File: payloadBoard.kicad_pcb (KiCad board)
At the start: 4 copper layers, 20 x 45 mm, 49 parts, among them J1 USB_C_Receptacle_USB2.0_16P, J2 SERVO, J3 2S Battery, J4 Conn_01x04, U1 nRF52833_QDxx, U2 AT25SF041-SSHB-X, U3 LSM6DSO32, U4 AP63205WU, U5 AP63203WU, Y2 Crystal_GND24

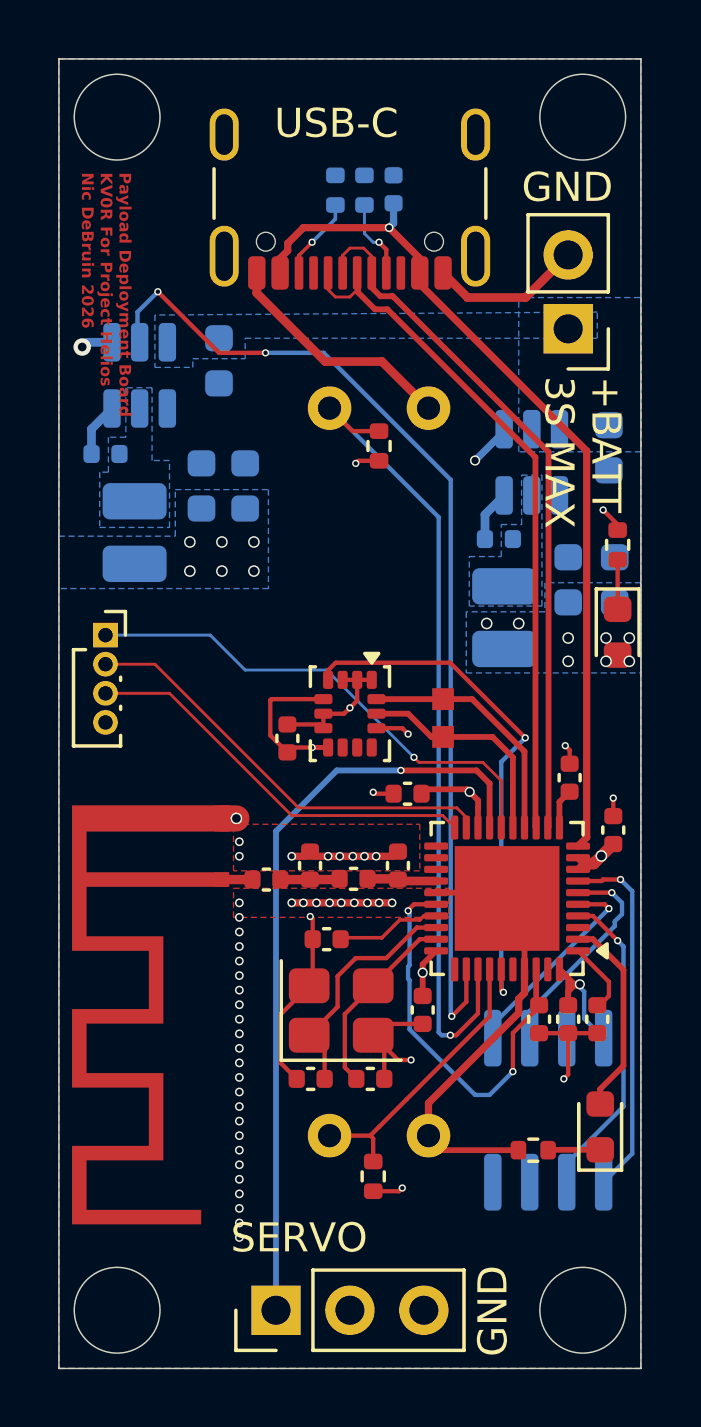
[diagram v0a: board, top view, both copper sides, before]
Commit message: board done, plenty small
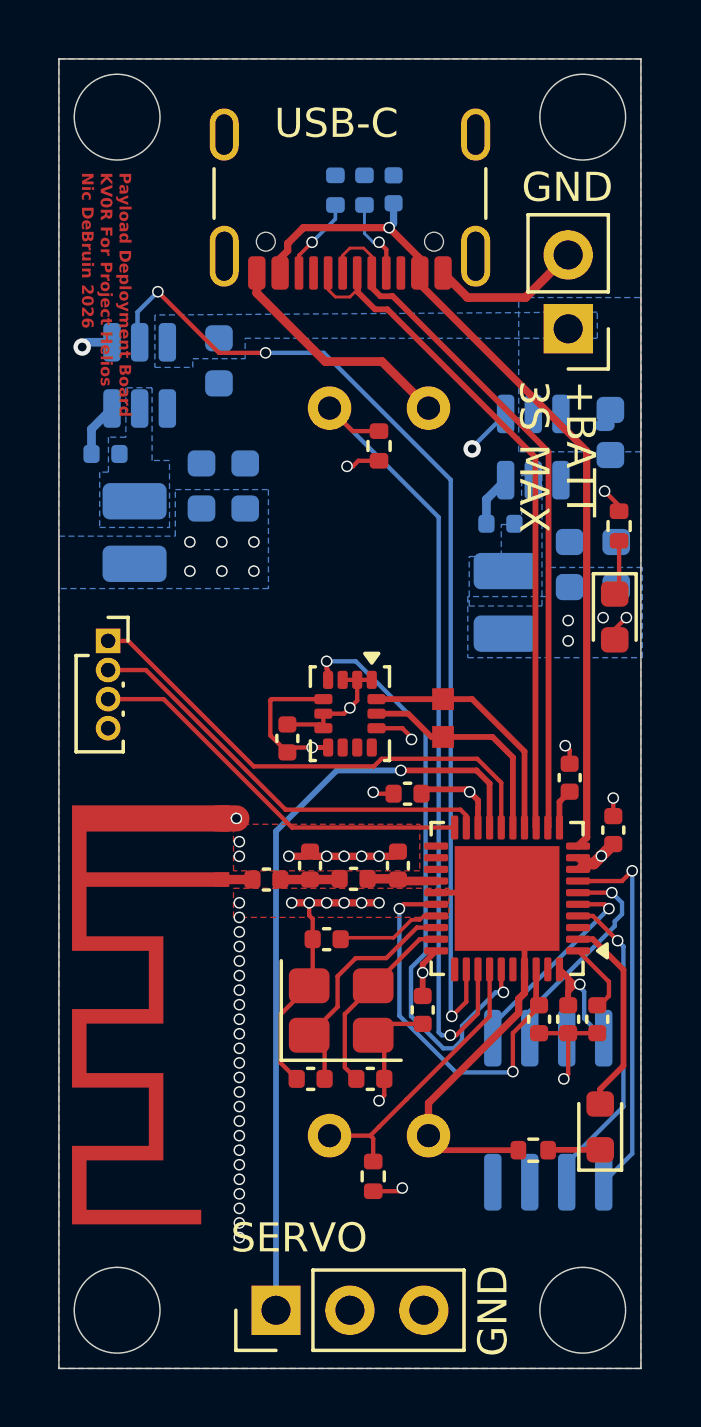
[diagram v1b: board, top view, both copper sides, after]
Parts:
- moved R7 0.65 mm to (164.2, 81.1)
- moved D1 0.53 mm to (164.1, 84.2)
- moved C20 0.53 mm to (164.2, 82.4)
- moved C21 0.53 mm to (162.6, 82.4)
- moved C19 0.53 mm to (160.2, 81.0)
- moved L4 0.53 mm to (160.3, 83.7)
- moved U5 0.53 mm to (161.3, 78.3)
- moved C18 0.53 mm to (163.9, 77.8)
- moved J4 0.22 mm to (146.7, 85.0)
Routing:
- net IMU_IRQ1: track 18.2 -> 20.6 mm
- net GND: track 59.1 -> 58.1 mm, vias 50 -> 45
- net +3.3V: track 23.9 -> 24.6 mm, vias 17 -> 13
- net CS: track 12.5 -> 13.1 mm
- net Net-(J4-Pin_1): vias 1 -> 0
